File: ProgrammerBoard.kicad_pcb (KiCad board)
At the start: 2 copper layers, 12 parts, among them IC1 FT232RL, J1 USB_B_Micro, J2 Jumper_For_RJ45

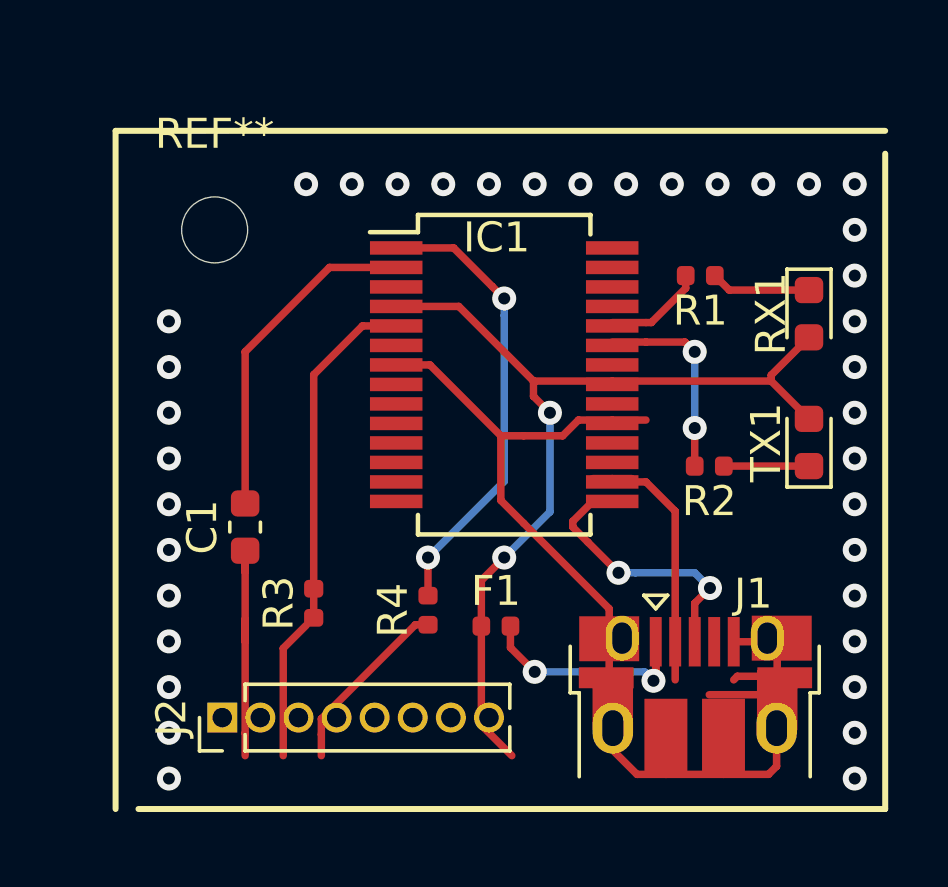
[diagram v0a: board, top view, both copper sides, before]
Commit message: Finished Rev 0.0.1
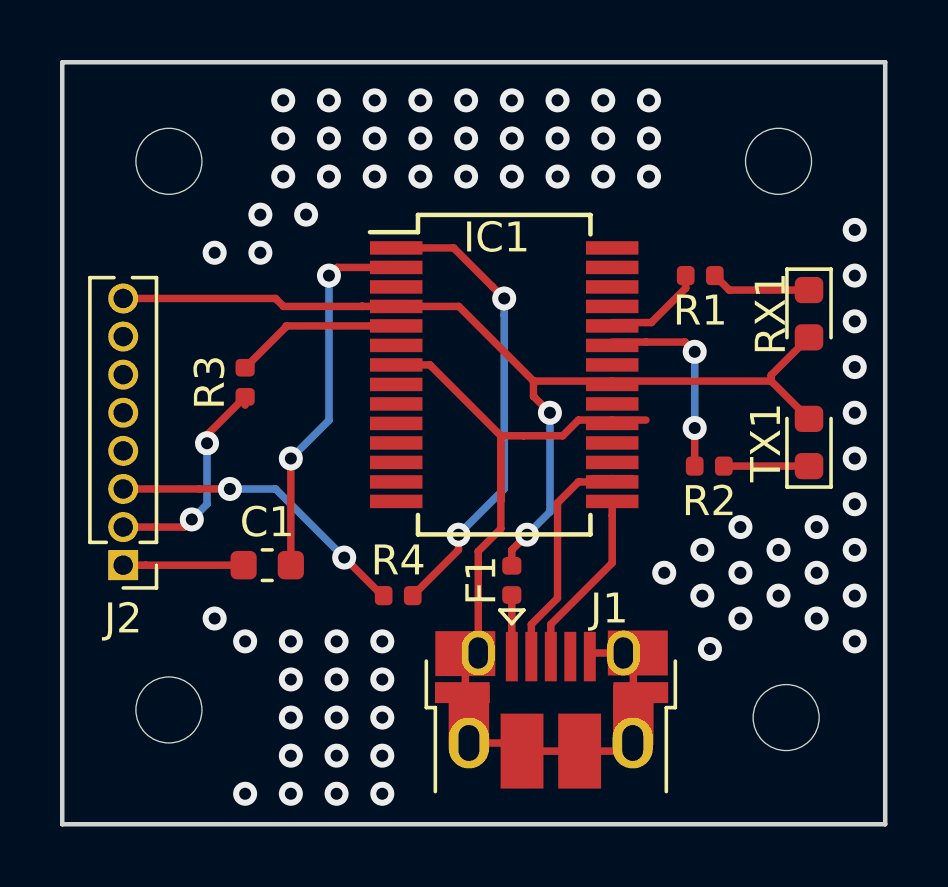
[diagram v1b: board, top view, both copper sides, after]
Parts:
- added ?: MountingHole_2.2mm_M2, MountingHole:MountingHole_2.2mm_M2, F.Cu at (80.5, 56.6)
- added ?: MountingHole_2.2mm_M2, MountingHole:MountingHole_2.2mm_M2, F.Cu at (59.9, 56.4)
- added ?: MountingHole_2.2mm_M2, MountingHole:MountingHole_2.2mm_M2, F.Cu at (80.3, 38.1)
- added G***: LOGO, Libraries:LOGO_black, B.Cu at (70.9, 46.2)
- moved R3 7.71 mm to (62.5, 45.5)
- moved J2 6.06 mm to (58.4, 51.6), turned to 180 degrees
- moved J1 4.82 mm to (72.7, 56.4)
- moved ? 2.75 mm to (59.9, 38.1)
- moved F1 1.61 mm to (71.4, 52.1), turned to 270 degrees
- moved C1 1.47 mm to (63.2, 51.6), turned to 0 degrees
- moved R4 1.11 mm to (67.6, 52.6), turned to 0 degrees
- renumbered REF** to ?
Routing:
- net Earth: track 39.5 -> 29.3 mm
- net Net-(F1-Pad2): track 8.35 -> 2.05 mm, vias 2 -> 0
- net Net-(IC1-Pad5): track 11.3 -> 5.63 mm
- net Net-(C1-Pad1): track 8.11 -> 4.01 mm
- net Net-(J2-Pad3): track 6.08 -> 10.2 mm, vias 0 -> 2
- net Net-(J2-Pad2): track 4.66 -> 7.49 mm, vias 0 -> 2
- net Net-(IC1-Pad15): track 9.49 -> 6.67 mm, vias 2 -> 0
- net +5V: track 31.4 -> 33.4 mm
- net Net-(C1-Pad2): track 11.3 -> 12.5 mm, vias 0 -> 2
- net GNDREF: vias 37 -> 71
- added copper zone on B.Cu, net GNDREF
- added copper zone on F.Cu, net GNDREF
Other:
- board outline added: 27.4 x 25.4 mm
- board text added: "Programmer Board Created by Jack Kufa For MST URT"
- board text added: "Rev 0.0.1 Rev Date 10-10-18"
